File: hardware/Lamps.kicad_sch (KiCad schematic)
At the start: 3 parts

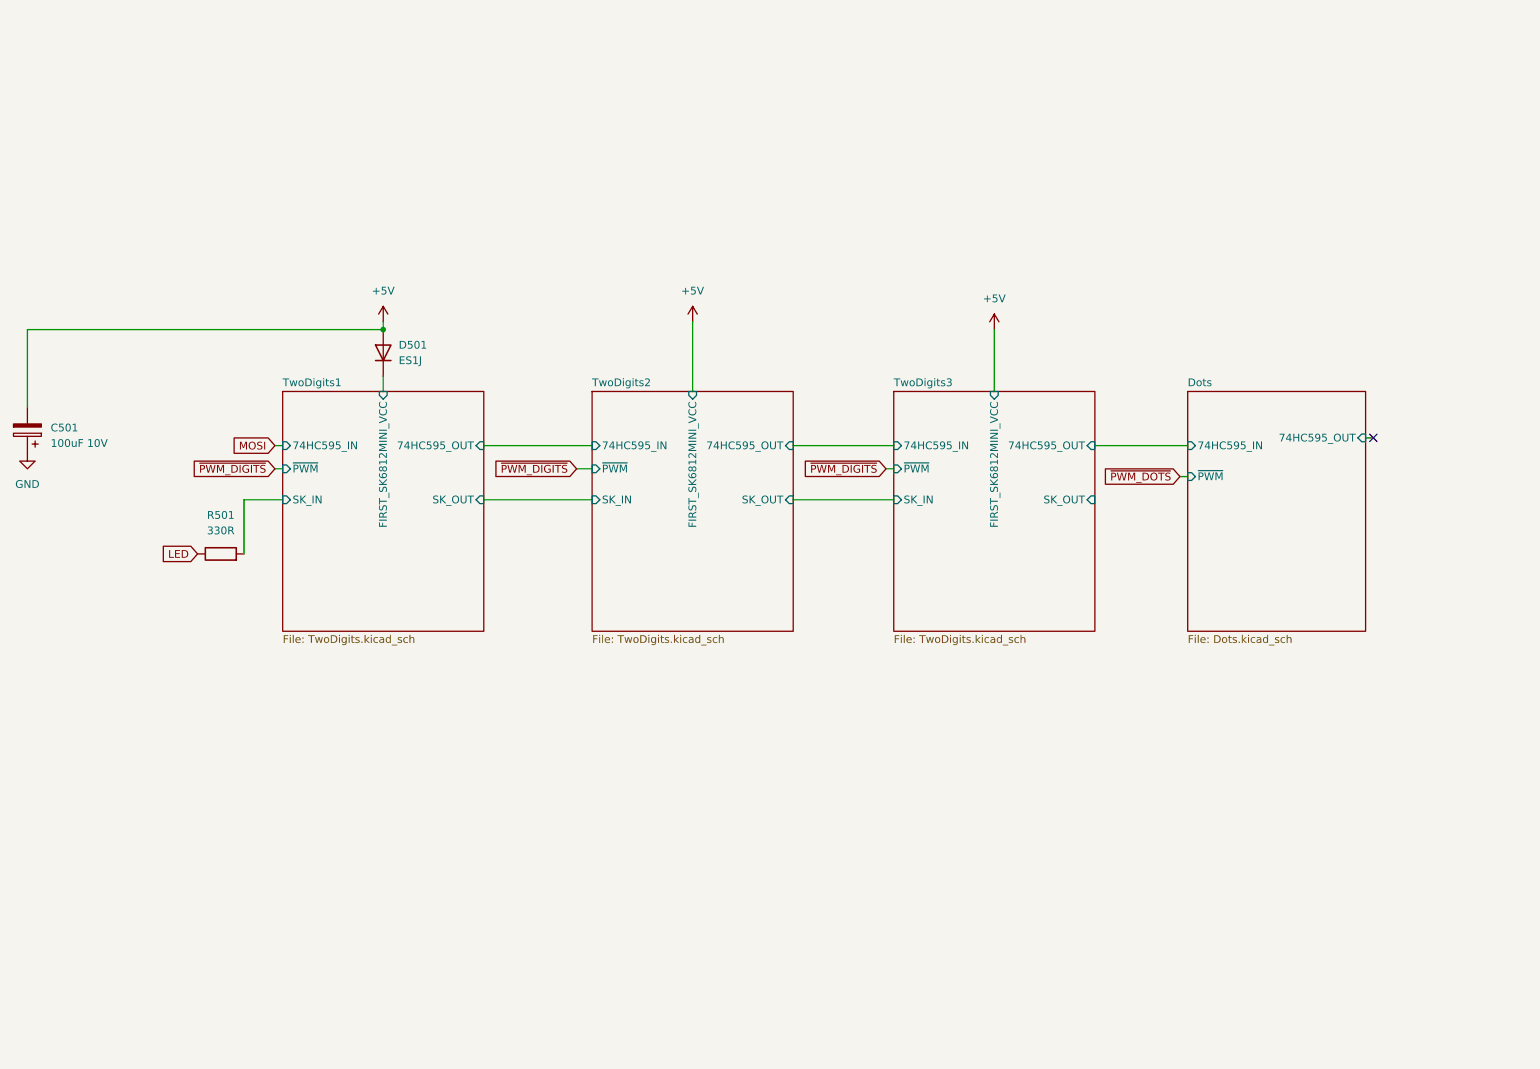
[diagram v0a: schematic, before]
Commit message: 2/static version
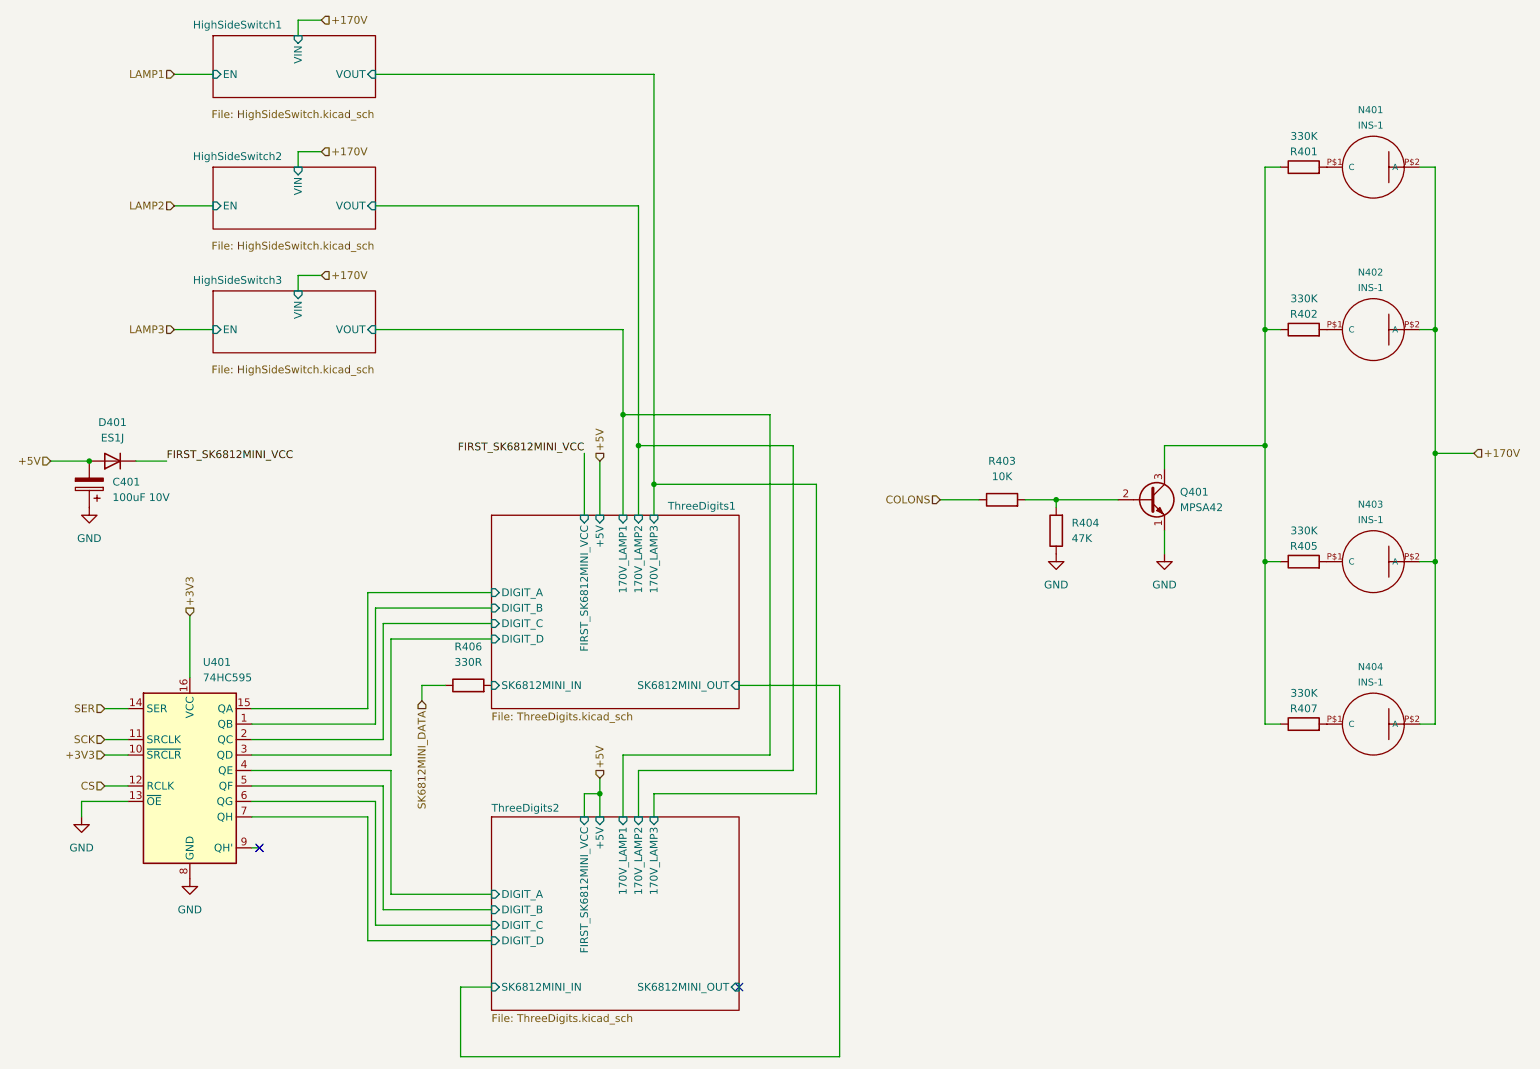
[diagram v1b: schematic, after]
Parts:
- removed C501: 100uF 10V, Capacitor_THT:CP_Radial_D6.3mm_P2.50mm, symbol Device:C_Polarized
- removed D501: ES1J, Diode_SMD:D_SMA_Handsoldering, symbol Device:D
- removed R501: 330R, Resistor_SMD:R_0603_1608Metric, symbol Device:R
- added C401: 100uF 10V, Capacitor_THT:CP_Radial_D6.3mm_P2.50mm, symbol Device:C_Polarized
- added D401: ES1J, Diode_SMD:D_SMA, symbol Device:D
- added N401, N402, N403, N404: INS-1, mynixies:mynixies-INS-1, symbol mynixies:INS-1
- added Q401: MPSA42, Package_TO_SOT_THT:TO-92_Inline, symbol Transistor_BJT:MPSA42
- added R401, R402, R405, R407: 330K, Resistor_SMD:R_1206_3216Metric, symbol Device:R
- added R403: 10K, Resistor_SMD:R_0603_1608Metric, symbol Device:R
- added R404: 47K, Resistor_SMD:R_0603_1608Metric, symbol Device:R
- added R406: 330R, Resistor_SMD:R_0603_1608Metric, symbol Device:R
- added U401: 74HC595, Package_SO:TSSOP-16_4.4x5mm_P0.65mm, symbol 74xx:74HC595
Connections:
- net +5V: now also C401.2, D401.2 (A)
- net GND: now also C401.1, Q401.1 (E), R404.1, U401.13 (~{OE}), U401.8 (GND)
- new net: Q401.3 (C), R401.1, R402.1, R405.1, R407.1
- new net: N401.P$1 (C), R401.2
- new net: Q401.2 (B), R403.2, R404.2
- new net: N403.P$1 (C), R405.2
- new net: N404.P$1 (C), R407.2
- new net: N402.P$1 (C), R402.2
- new net +170V: N401.P$2 (A), N402.P$2 (A), N403.P$2 (A), N404.P$2 (A)
- new net +3V3: U401.10 (~{SRCLR}), U401.16 (VCC)
- new net COLONS: R403.1
- new net CS: U401.12 (RCLK)
- new net FIRST_SK6812MINI_VCC: D401.1 (K)
- new net SCK: U401.11 (SRCLK)
- new net SER: U401.14 (SER)
- new net SK6812MINI_DATA: R406.1
- new net ThreeDigits1/DIGIT_A: U401.15 (QA)
- new net ThreeDigits1/DIGIT_B: U401.1 (QB)
- new net ThreeDigits1/DIGIT_C: U401.2 (QC)
- new net ThreeDigits1/DIGIT_D: U401.3 (QD)
- new net ThreeDigits1/SK6812MINI_IN: R406.2
- new net ThreeDigits2/DIGIT_A: U401.4 (QE)
- new net ThreeDigits2/DIGIT_B: U401.5 (QF)
- new net ThreeDigits2/DIGIT_C: U401.6 (QG)
- new net ThreeDigits2/DIGIT_D: U401.7 (QH)
- no-connect marks 1 -> 2
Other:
- removed sheet Dots
- removed sheet TwoDigits1
- removed sheet TwoDigits2
- removed sheet TwoDigits3
- added sheet HighSideSwitch1 (HighSideSwitch.kicad_sch)
- added sheet HighSideSwitch2 (HighSideSwitch.kicad_sch)
- added sheet HighSideSwitch3 (HighSideSwitch.kicad_sch)
- added sheet ThreeDigits1 (ThreeDigits.kicad_sch)
- added sheet ThreeDigits2 (ThreeDigits.kicad_sch)
